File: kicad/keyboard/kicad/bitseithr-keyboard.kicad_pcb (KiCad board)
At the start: 2 copper layers, 365 x 206 mm, 103 parts, among them P2 KEYB CONN 1

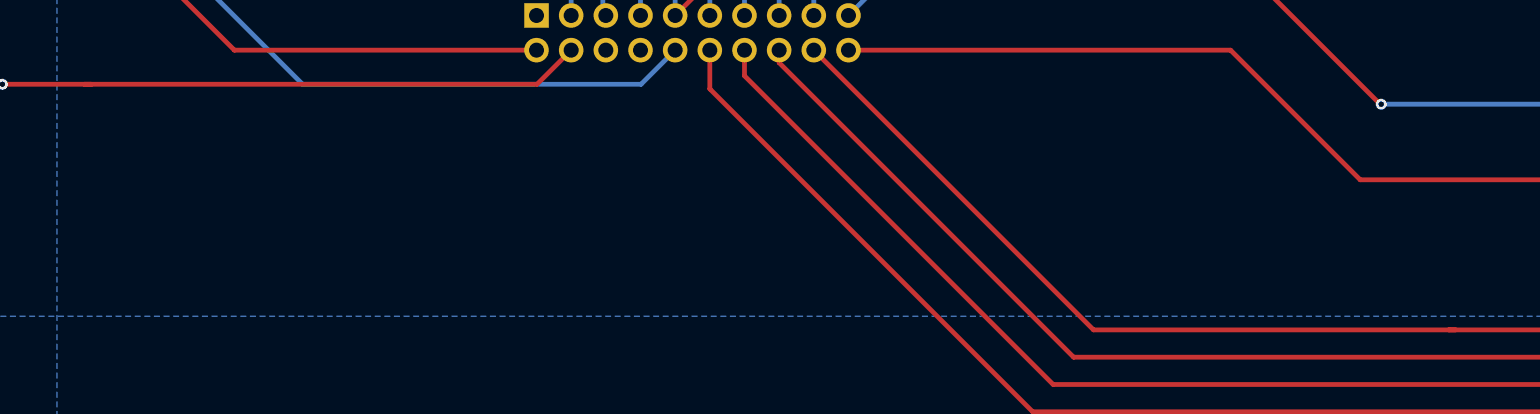
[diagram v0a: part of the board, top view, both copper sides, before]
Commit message: drc fixes
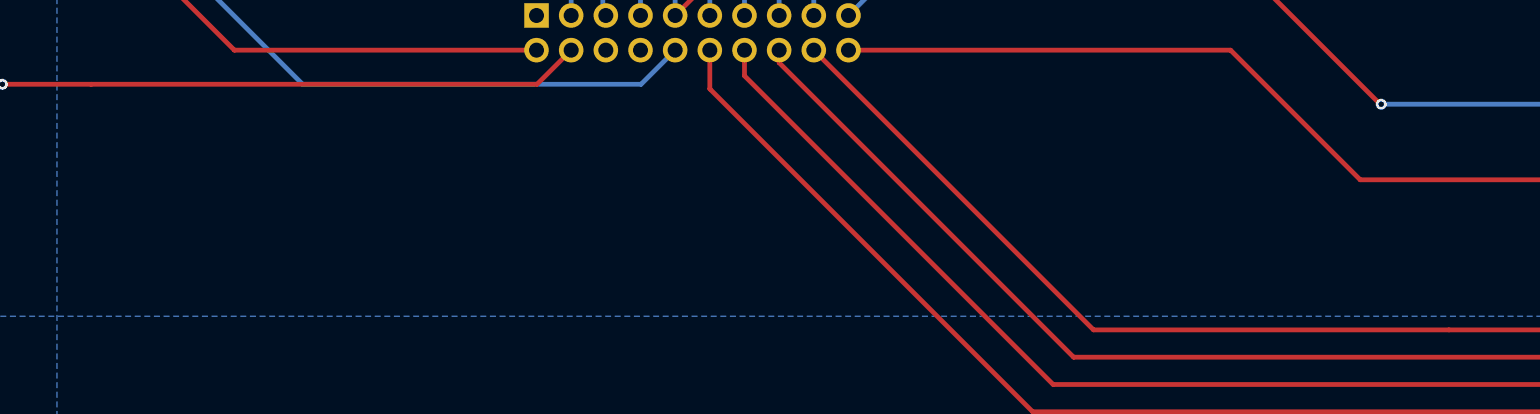
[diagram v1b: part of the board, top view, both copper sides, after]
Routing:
- net ROW4: track 405.5 -> 405.0 mm
- net GND: track 217.0 -> 216.5 mm
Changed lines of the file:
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@@
-	(segment
-		(start 154 240)
-		(end 154.5 240)
-		(width 0.35)
-		(layer "F.Cu")
-		(net 9)
-	)
 	(segment
 		(start 154 240)
@@
 		(width 0.35)
 		(layer "F.Cu")
-		(net 42)
-	)
-	(segment
-		(start 54.5 222)
-		(end 54 222)
-		(width 0.35)
-		(layer "F.Cu")
